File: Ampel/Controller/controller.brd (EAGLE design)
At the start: 31.7 x 33.7 mm, 8 parts, among them IC1 ATtiny25

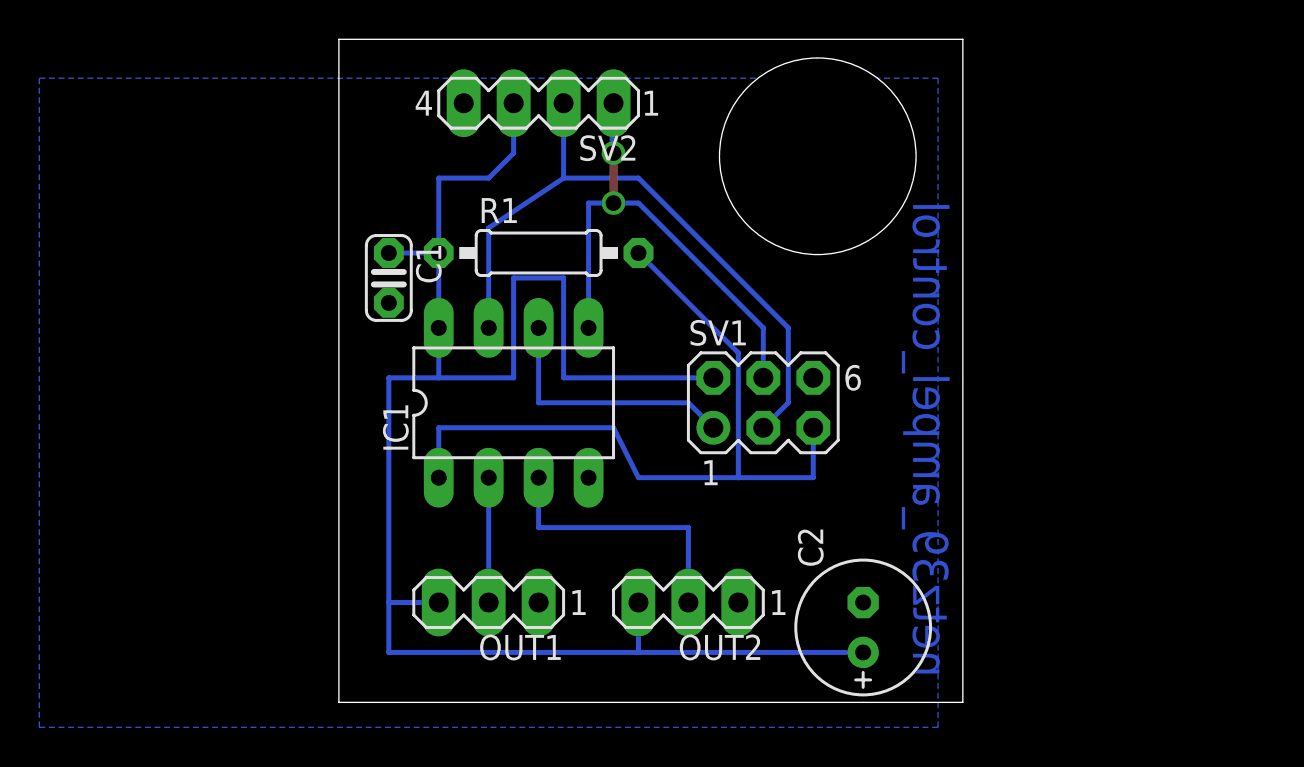
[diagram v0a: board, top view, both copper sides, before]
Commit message: letzte Anpassungen zum Ätzen
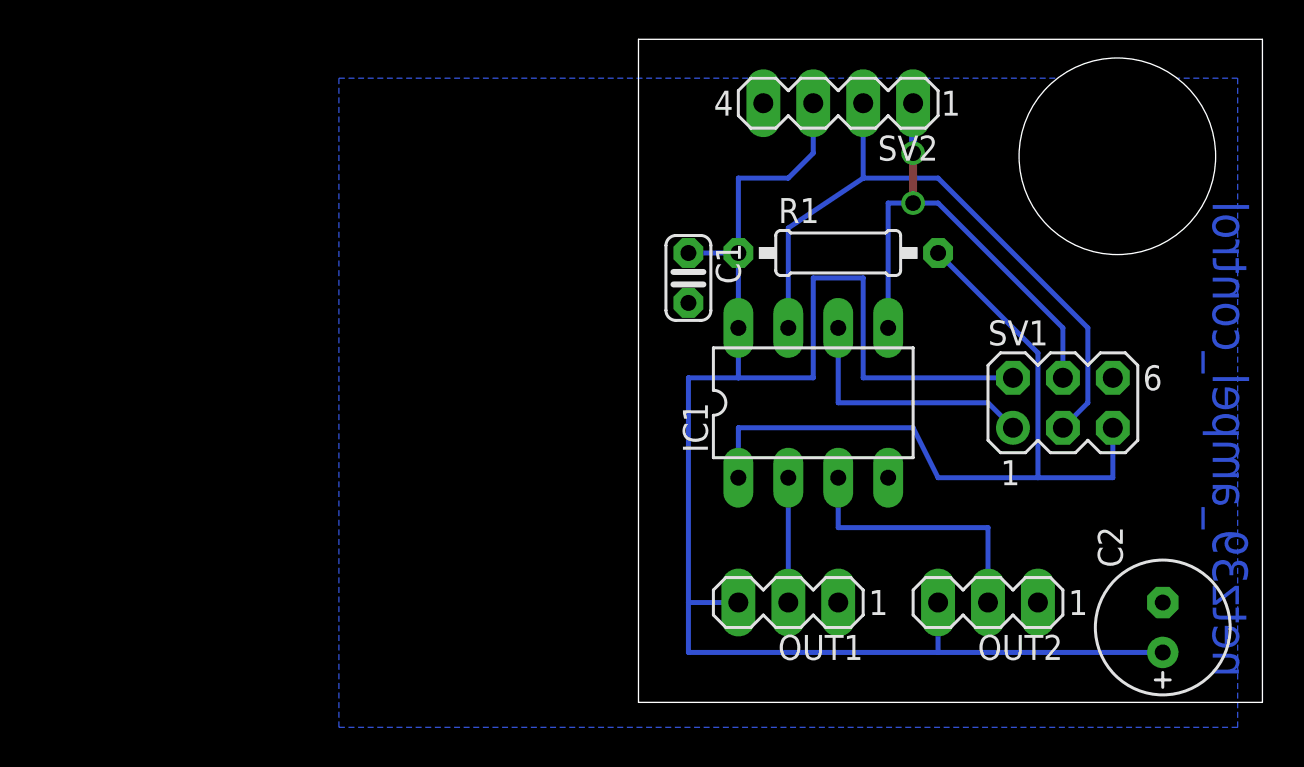
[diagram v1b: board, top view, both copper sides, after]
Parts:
- moved C1 15.2 mm to (17.8, 21.6)
- moved OUT2 15.2 mm to (33.0, 5.08)
- moved IC1 15.2 mm to (24.1, 15.2)
- moved OUT1 15.2 mm to (22.9, 5.08)
- moved R1 15.2 mm to (25.4, 22.9)
- moved SV1 15.2 mm to (36.8, 15.2)
- moved SV2 15.2 mm to (25.4, 30.5)
- moved C2 15.2 mm to (41.9, 3.81)
